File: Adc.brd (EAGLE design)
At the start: 120.6 x 100 mm, 97 parts, among them IC1 ADS1256IDBT, IC10 AD8605ARTZ, IC11 REF3125AIDBZT, IC12 MCP170333MB, IC2 ADUM1402ARWZ, IC3 AD8605ARTZ, IC4 AD8605ARTZ, IC5 AD8605ARTZ, IC6 AD8605ARTZ, IC7 AD8605ARTZ, IC8 AD8605ARTZ, IC9 AD8605ARTZ, Q1 8MHz

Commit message: Rename lbr
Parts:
- G1: device nanoeeg:TMV0505D -> femtoexg:TMV0505D
- IC1: device nanoeeg:ADS1256IDBT -> femtoexg:ADS1256IDBT
- IC10, IC3, IC4, IC5, IC6, IC7, IC8, IC9: device nanoeeg:AD8605ARTZ -> femtoexg:AD8605ARTZ
- IC11: device nanoeeg:REF3125AIDBZT -> femtoexg:REF3125AIDBZT
- IC2: device nanoeeg:ADUM1402ARWZ -> femtoexg:ADUM1402ARWZ
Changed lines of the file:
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@@
 </autorouter>
 <elements>
-<element name="IC1" library="nanoeeg" package="ADS1256IDBT" value="ADS1256IDBT" x="29.21" y="48.26"/>
-<element name="IC2" library="nanoeeg" package="ADUM1402ARWZ" value="ADUM1402ARWZ" x="60.96" y="71.12"/>
-<element name="G1" library="nanoeeg" package="TMV0505D" value="TMV0505D" x="82.55" y="91.44" rot="R270"/>
-<element name="IC3" library="nanoeeg" package="AD8605ARTZ" value="AD8605ARTZ" x="20.32" y="21.59" rot="R180"/>
+<element name="IC1" library="femtoexg" package="ADS1256IDBT" value="ADS1256IDBT" x="29.21" y="48.26"/>
+<element name="IC2" library="femtoexg" package="ADUM1402ARWZ" value="ADUM1402ARWZ" x="60.96" y="71.12"/>
+<element name="G1" library="femtoexg" package="TMV0505D" value="TMV0505D" x="82.55" y="91.44" rot="R270"/>
+<element name="IC3" library="femtoexg" package="AD8605ARTZ" value="AD8605ARTZ" x="20.32" y="21.59" rot="R180"/>
 <element name="C1" library="rcl" package="C0805" value="0.1uF" x="19.05" y="26.67" rot="R270"/>
 <element name="C2" library="rcl" package="C0805" value="0.1uF" x="21.59" y="26.67" rot="R90"/>
@@
 <element name="C3" library="rcl" package="C0805" value="0.1uF" x="20.32" y="33.02" rot="R270"/>
 <element name="JP1" library="pinhead" package="1X04" value="" x="16.51" y="8.89" rot="R270"/>
-<element name="IC4" library="nanoeeg" package="AD8605ARTZ" value="AD8605ARTZ" x="30.48" y="21.59" rot="R180"/>
+<element name="IC4" library="femtoexg" package="AD8605ARTZ" value="AD8605ARTZ" x="30.48" y="21.59" rot="R180"/>
 <element name="C4" library="rcl" package="C0805" value="0.1uF" x="29.21" y="26.67" rot="R270"/>
 <element name="C5" library="rcl" package="C0805" value="0.1uF" x="31.75" y="26.67" rot="R90"/>
@@
 <element name="C6" library="rcl" package="C0805" value="0.1uF" x="30.48" y="33.02" rot="R270"/>
 <element name="JP2" library="pinhead" package="1X04" value="" x="26.67" y="8.89" rot="R270"/>
-<element name="IC5" library="nanoeeg" package="AD8605ARTZ" value="AD8605ARTZ" x="40.64" y="21.59" rot="R180"/>
+<element name="IC5" library="femtoexg" package="AD8605ARTZ" value="AD8605ARTZ" x="40.64" y="21.59" rot="R180"/>
 <element name="C7" library="rcl" package="C0805" value="0.1uF" x="39.37" y="26.67" rot="R270"/>
 <element name="C8" library="rcl" package="C0805" value="0.1uF" x="41.91" y="26.67" rot="R90"/>
@@
 <element name="C9" library="rcl" package="C0805" value="0.1uF" x="40.64" y="33.02" rot="R270"/>
 <element name="JP3" library="pinhead" package="1X04" value="" x="36.83" y="8.89" rot="R270"/>
-<element name="IC6" library="nanoeeg" package="AD8605ARTZ" value="AD8605ARTZ" x="50.8" y="21.59" rot="R180"/>
+<element name="IC6" library="femtoexg" package="AD8605ARTZ" value="AD8605ARTZ" x="50.8" y="21.59" rot="R180"/>
 <element name="C10" library="rcl" package="C0805" value="0.1uF" x="49.53" y="26.67" rot="R270"/>
 <element name="C11" library="rcl" package="C0805" value="0.1uF" x="52.07" y="26.67" rot="R90"/>
@@
 <element name="C12" library="rcl" package="C0805" value="0.1uF" x="50.8" y="33.02" rot="R270"/>
 <element name="JP4" library="pinhead" package="1X04" value="" x="46.99" y="8.89" rot="R270"/>
-<element name="IC7" library="nanoeeg" package="AD8605ARTZ" value="AD8605ARTZ" x="60.96" y="21.59" rot="R180"/>
+<element name="IC7" library="femtoexg" package="AD8605ARTZ" value="AD8605ARTZ" x="60.96" y="21.59" rot="R180"/>
 <element name="C13" library="rcl" package="C0805" value="0.1uF" x="59.69" y="26.67" rot="R270"/>
 <element name="C14" library="rcl" package="C0805" value="0.1uF" x="62.23" y="26.67" rot="R90"/>
@@
 <element name="C15" library="rcl" package="C0805" value="0.1uF" x="60.96" y="33.02" rot="R270"/>
 <element name="JP5" library="pinhead" package="1X04" value="" x="57.15" y="8.89" rot="R270"/>
-<element name="IC8" library="nanoeeg" package="AD8605ARTZ" value="AD8605ARTZ" x="71.12" y="21.59" rot="R180"/>
+<element name="IC8" library="femtoexg" package="AD8605ARTZ" value="AD8605ARTZ" x="71.12" y="21.59" rot="R180"/>
 <element name="C16" library="rcl" package="C0805" value="0.1uF" x="69.85" y="26.67" rot="R270"/>
 <element name="C17" library="rcl" package="C0805" value="0.1uF" x="72.39" y="26.67" rot="R90"/>
@@
 <element name="C18" library="rcl" package="C0805" value="0.1uF" x="71.12" y="33.02" rot="R270"/>
 <element name="JP6" library="pinhead" package="1X04" value="" x="67.31" y="8.89" rot="R270"/>
-<element name="IC9" library="nanoeeg" package="AD8605ARTZ" value="AD8605ARTZ" x="81.28" y="21.59" rot="R180"/>
+<element name="IC9" library="femtoexg" package="AD8605ARTZ" value="AD8605ARTZ" x="81.28" y="21.59" rot="R180"/>
 <element name="C19" library="rcl" package="C0805" value="0.1uF" x="80.01" y="26.67" rot="R270"/>
 <element name="C20" library="rcl" package="C0805" value="0.1uF" x="82.55" y="26.67" rot="R90"/>
@@
 <element name="C21" library="rcl" package="C0805" value="0.1uF" x="81.28" y="33.02" rot="R270"/>
 <element name="JP7" library="pinhead" package="1X04" value="" x="77.47" y="8.89" rot="R270"/>
-<element name="IC10" library="nanoeeg" package="AD8605ARTZ" value="AD8605ARTZ" x="91.44" y="21.59" rot="R180"/>
+<element name="IC10" library="femtoexg" package="AD8605ARTZ" value="AD8605ARTZ" x="91.44" y="21.59" rot="R180"/>
 <element name="C22" library="rcl" package="C0805" value="0.1uF" x="90.17" y="26.67" rot="R270"/>
 <element name="C23" library="rcl" package="C0805" value="0.1uF" x="92.71" y="26.67" rot="R90"/>
@@
 <element name="C27" library="rcl" package="C0805" value="0.1uF" x="33.02" y="54.61" rot="R180"/>
 <element name="C28" library="rcl" package="E2-4" value="47uF" x="33.02" y="62.23"/>
-<element name="IC11" library="nanoeeg" package="REF3125AIDBZT" value="REF3125AIDBZT" x="34.29" y="71.12"/>
+<element name="IC11" library="femtoexg" package="REF3125AIDBZT" value="REF3125AIDBZT" x="34.29" y="71.12"/>
 <element name="Q1" library="crystal" package="HC49U-V" value="8MHz" x="21.59" y="57.15" rot="R180">
 <attribute name="OC_NEWARK" value="unknown" x="21.59" y="57.15" size="1.778" layer="27" rot="R180" display="off"/>

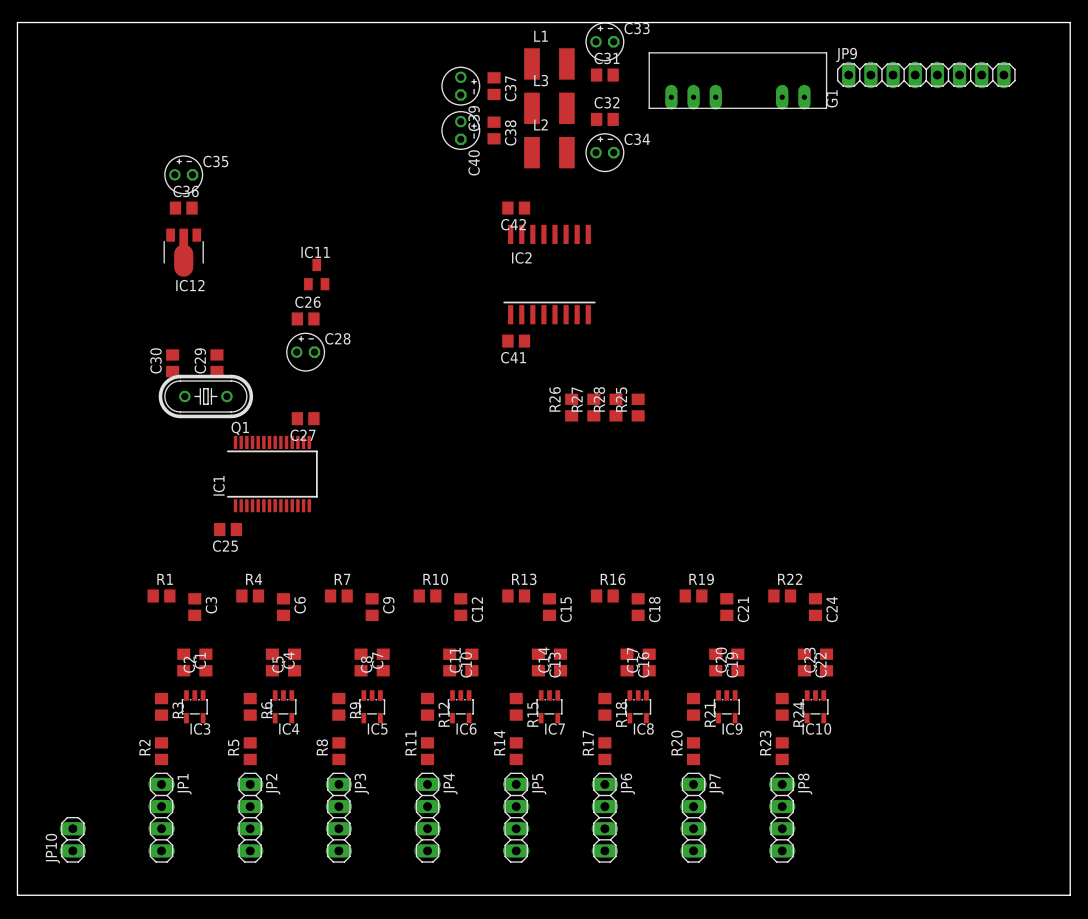
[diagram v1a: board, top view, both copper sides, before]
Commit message: Dimensions
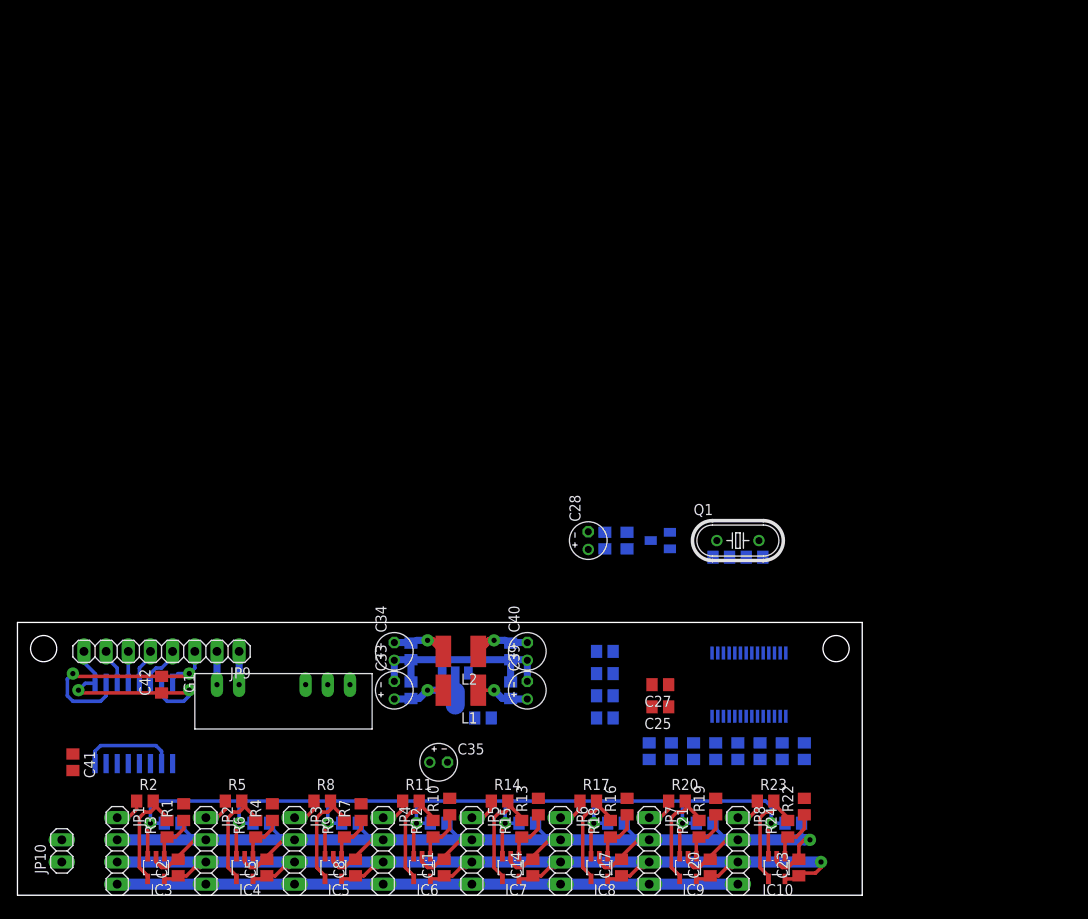
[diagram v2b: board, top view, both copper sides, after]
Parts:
- removed L3: (no value), rcl:L4532P
- added C43: 100pF, rcl:C0805
- moved JP9 109.7 mm to (16.5, 27.9), turned to 180 degrees
- moved G1 85.1 mm to (30.5, 24.1), turned to 90 degrees
- moved C33 78.1 mm to (43.2, 23.5), turned to 90 degrees
- moved C31 73.9 mm to (45.1, 23.5), flipped to the bottom, turned to 90 degrees
- moved C35 73.4 mm to (48.3, 15.2)
- moved L1 72.5 mm to (50.8, 23.5), turned to 180 degrees
- moved C3 71.8 mm to (90.2, 16.5), flipped to the bottom
- moved C30 70.3 mm to (84.5, 38.7), flipped to the bottom, turned to 0 degrees
- moved IC2 70.1 mm to (13.3, 19.7), flipped to the bottom
- moved C41 70.1 mm to (6.35, 15.2), turned to 270 degrees
- moved C39 69.6 mm to (58.4, 23.5), turned to 90 degrees
- moved C37 69.2 mm to (56.5, 23.5), flipped to the bottom, turned to 90 degrees
- moved C42 68.1 mm to (16.5, 24.1), turned to 90 degrees
- moved C36 67.7 mm to (53.3, 20.3), flipped to the bottom, turned to 180 degrees
- moved C32 64.9 mm to (45.1, 27.9), flipped to the bottom, turned to 90 degrees
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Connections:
- removed net GNDIO: C27.2, C29.2, C30.2, C31.2, C32.1, C33.-, C34.+, C35.-, C36.2, C41.1, G1.6, IC1.17, IC1.20, IC12.1, IC2.2, IC2.8, L3.2
- net GND: now also C27.2, C29.2, C30.2, C31.2, C32.1, C33.-, C34.+, C35.-, C36.2, C41.1, C43.2, G1.6, IC1.17, IC1.20, IC12.1, IC2.2, IC2.8; no longer L3.1
- net N$51: now also JP9.2; no longer JP9.1
- net N$52: now also JP9.1; no longer JP9.2
- net REF: now also C43.1
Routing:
- net GND: track 0.00 -> 201.2 mm, vias 0 -> 1
- net REF: track 0.00 -> 134.7 mm, vias 0 -> 8
- net +5VA: track 0.00 -> 131.0 mm, vias 0 -> 2
- net -5VA: track 0.00 -> 77.4 mm, vias 0 -> 1
- net N$43: track 0.00 -> 28.3 mm, vias 0 -> 2
- net N$40: track 0.00 -> 25.3 mm, vias 0 -> 2
- net N$29: track 0.00 -> 12.7 mm
- net N$9: track 0.00 -> 12.7 mm
- net N$5: track 0.00 -> 12.7 mm
- net N$17: track 0.00 -> 12.7 mm
- net N$1: track 0.00 -> 12.7 mm
- net N$21: track 0.00 -> 12.7 mm
- net N$13: track 0.00 -> 12.7 mm
- net N$25: track 0.00 -> 12.7 mm
- net N$41: track 0.00 -> 9.78 mm, vias 0 -> 1
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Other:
- board size 120.6 x 100 mm -> 96.8 x 31.3 mm
